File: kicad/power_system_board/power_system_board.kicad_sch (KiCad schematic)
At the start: 17 parts, among them J1 USB_B_Micro, U1 MCP73831-2-OT, U2 MCP73831-2-OT

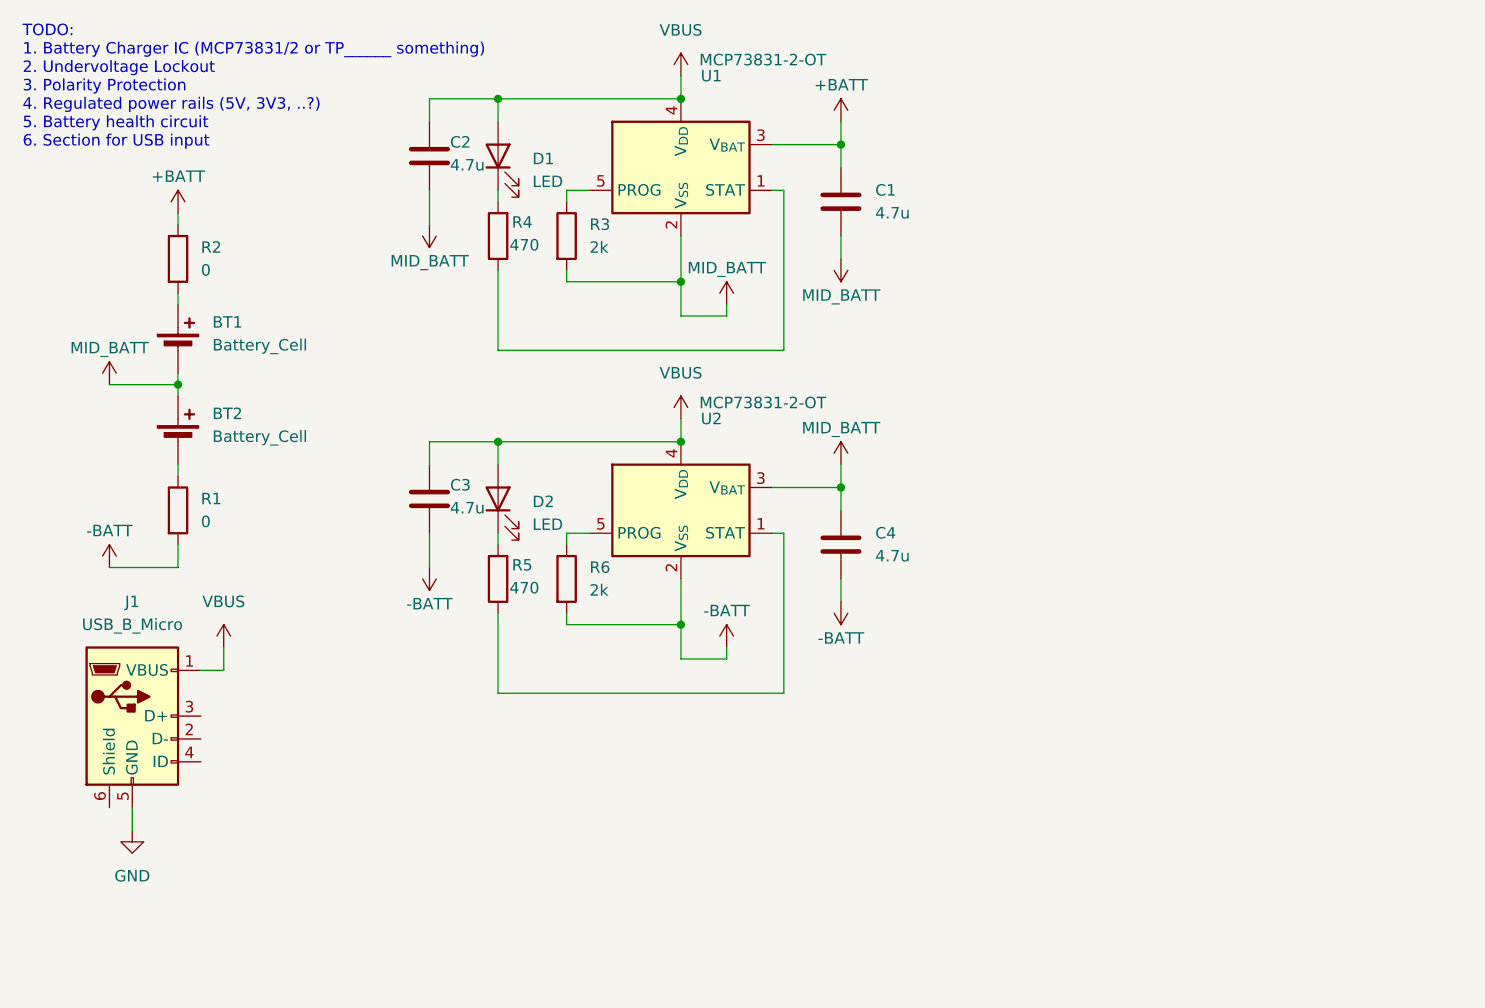
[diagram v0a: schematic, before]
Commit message: Big headway on the power module
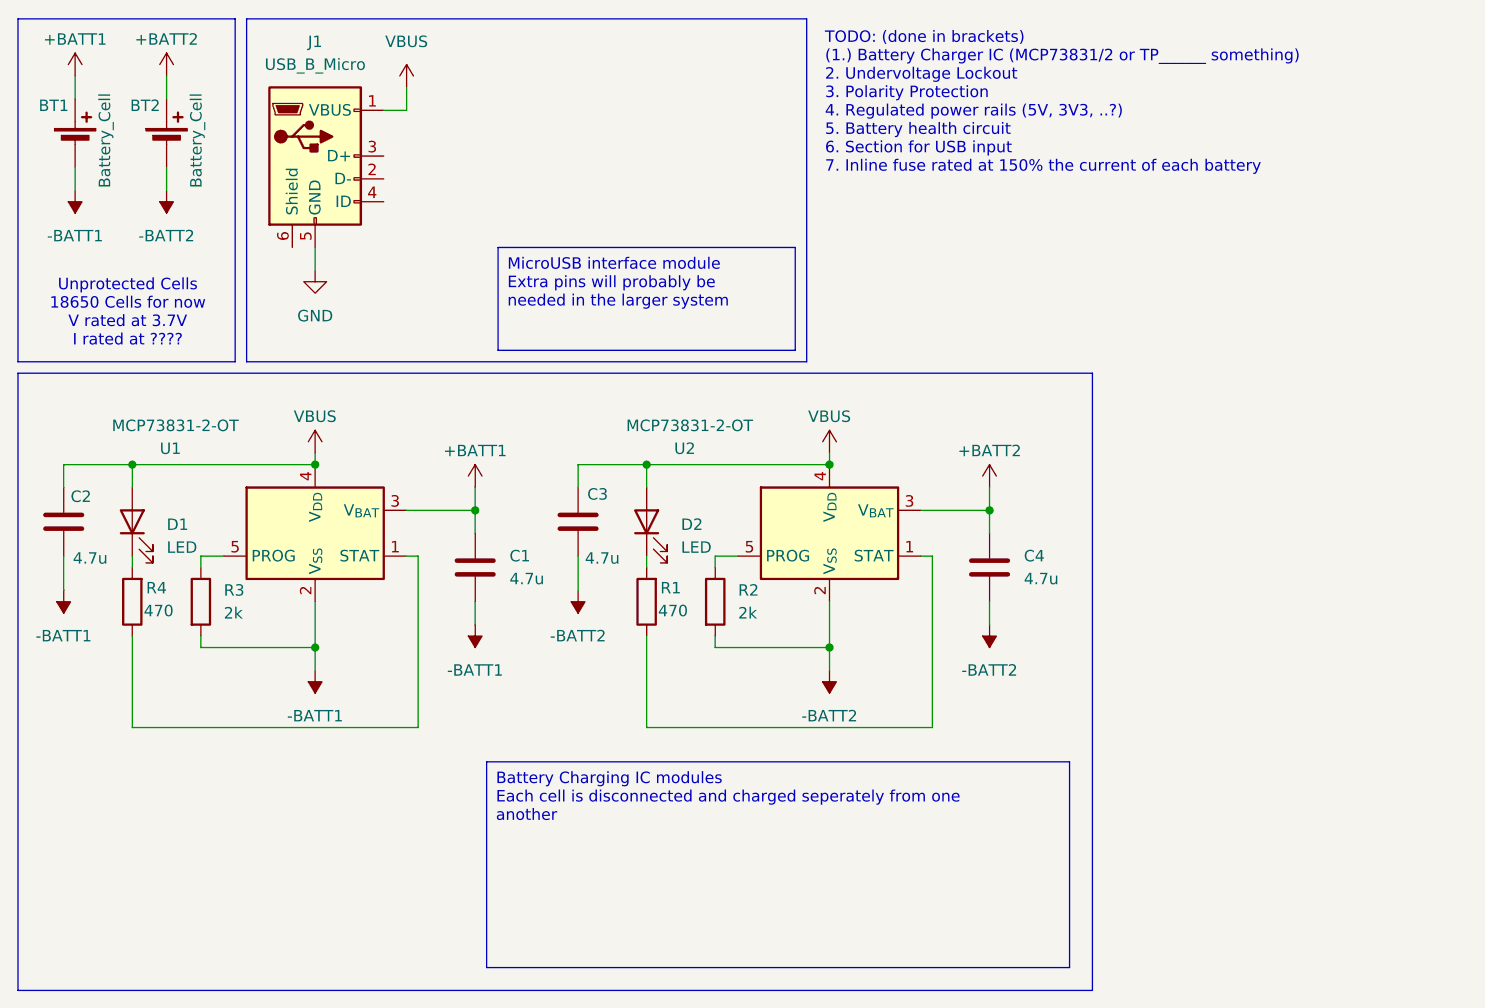
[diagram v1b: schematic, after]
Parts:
- removed R5: 470, symbol Device:R
- removed R6: 2k, symbol Device:R
- C1, C2, C3, C4: footprint (none) -> Capacitor_SMD:C_0805_2012Metric
- D1, D2: footprint (none) -> LED_SMD:LED_0805_2012Metric
- R1: value 0 -> 470; footprint (none) -> Resistor_SMD:R_0805_2012Metric
- R2: value 0 -> 2k
- R4: footprint (none) -> Resistor_SMD:R_0805_2012Metric
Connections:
- net VBUS: now also C2.1, C3.1; no longer C2.2, C3.2
- net at R1.1: now also U2.1 (STAT); no longer BT2.2 (-)
- net at U2.5 (PROG): now also R2.1
- net +BATT1: now reaches BT1.1 (+)
- net +BATT1: now also C1.1, U1.3 (V_{BAT}); no longer R2.2
- net at D2.1 (K): now also R1.2
- removed net +BATT: C1.1, R2.1, U1.3 (V_{BAT})
- net -BATT renamed -BATT2
- net -BATT2: now also BT2.2 (-), C3.2, R2.2; no longer C3.1, R1.2
- net MID_BATT renamed -BATT1
- net -BATT1: now also C2.2; no longer BT2.1 (+), C2.1, C4.1, U2.3 (V_{BAT})
- new net +BATT2: BT2.1 (+), C4.1, U2.3 (V_{BAT})
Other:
- note added: "TODO: (done in brackets) (1.) Battery Charger IC (MCP73831/2 or TP______ something) 2. Undervoltage Lockout 3. Polarity Protection 4. Regulated power rails (5V, 3V3, ..?) 5. Battery health circuit 6. Section for USB input 7. Inline fuse rated at 150% the current of each battery"
- note added: "Unprotected Cells 18650 Cells for now V rated at 3.7V I rated at ????"
- note removed: "TODO: 1. Battery Charger IC (MCP73831/2 or TP______ something) 2. Undervoltage Lockout 3. Polarity Protection 4. Regulated power rails (5V, 3V3, ..?) 5. Battery health circuit 6. Section for USB input"
- moved on the sheet: BT1, C1, D1, J1, R3, R4, U1
